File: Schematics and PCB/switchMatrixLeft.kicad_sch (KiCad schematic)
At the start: 151 parts, among them SW1 ESC, SW10 2, SW11 3, SW12 4, SW13 5, SW14 6, SW15 TAB, SW16 Q, SW17 W, SW18 E, SW19 R, SW2 F1, SW20 T, SW21 MAYUS, SW22 A, SW23 S, SW24 D, SW25 F, SW26 G, SW27 L_SHIFT, SW28 Z, SW29 X, SW3 F2, SW30 C, SW31 V, SW32 B, SW33 L_CRTL, SW34 OS, SW35 L_ALT, SW36 L_SPACE, SW4 F3, SW5 F4, SW6 F5, SW7 F6, SW8 `, SW9 1

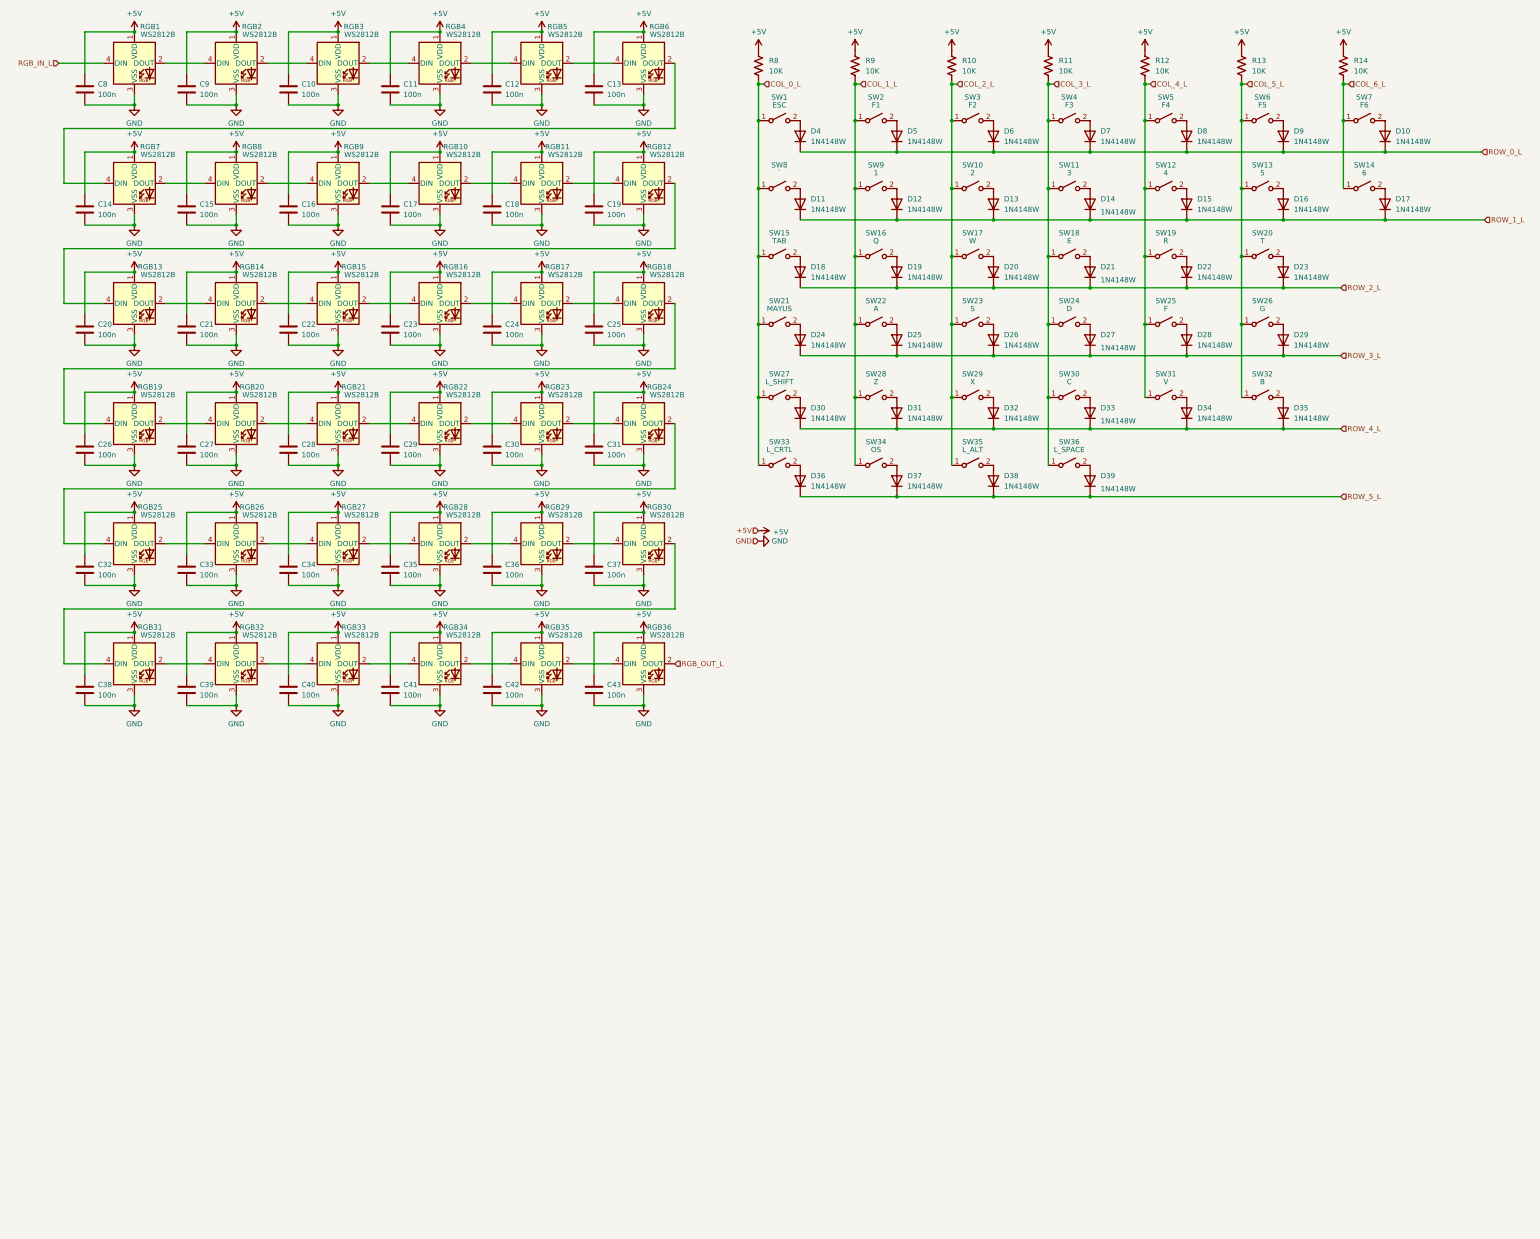
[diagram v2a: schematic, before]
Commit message: minor changes
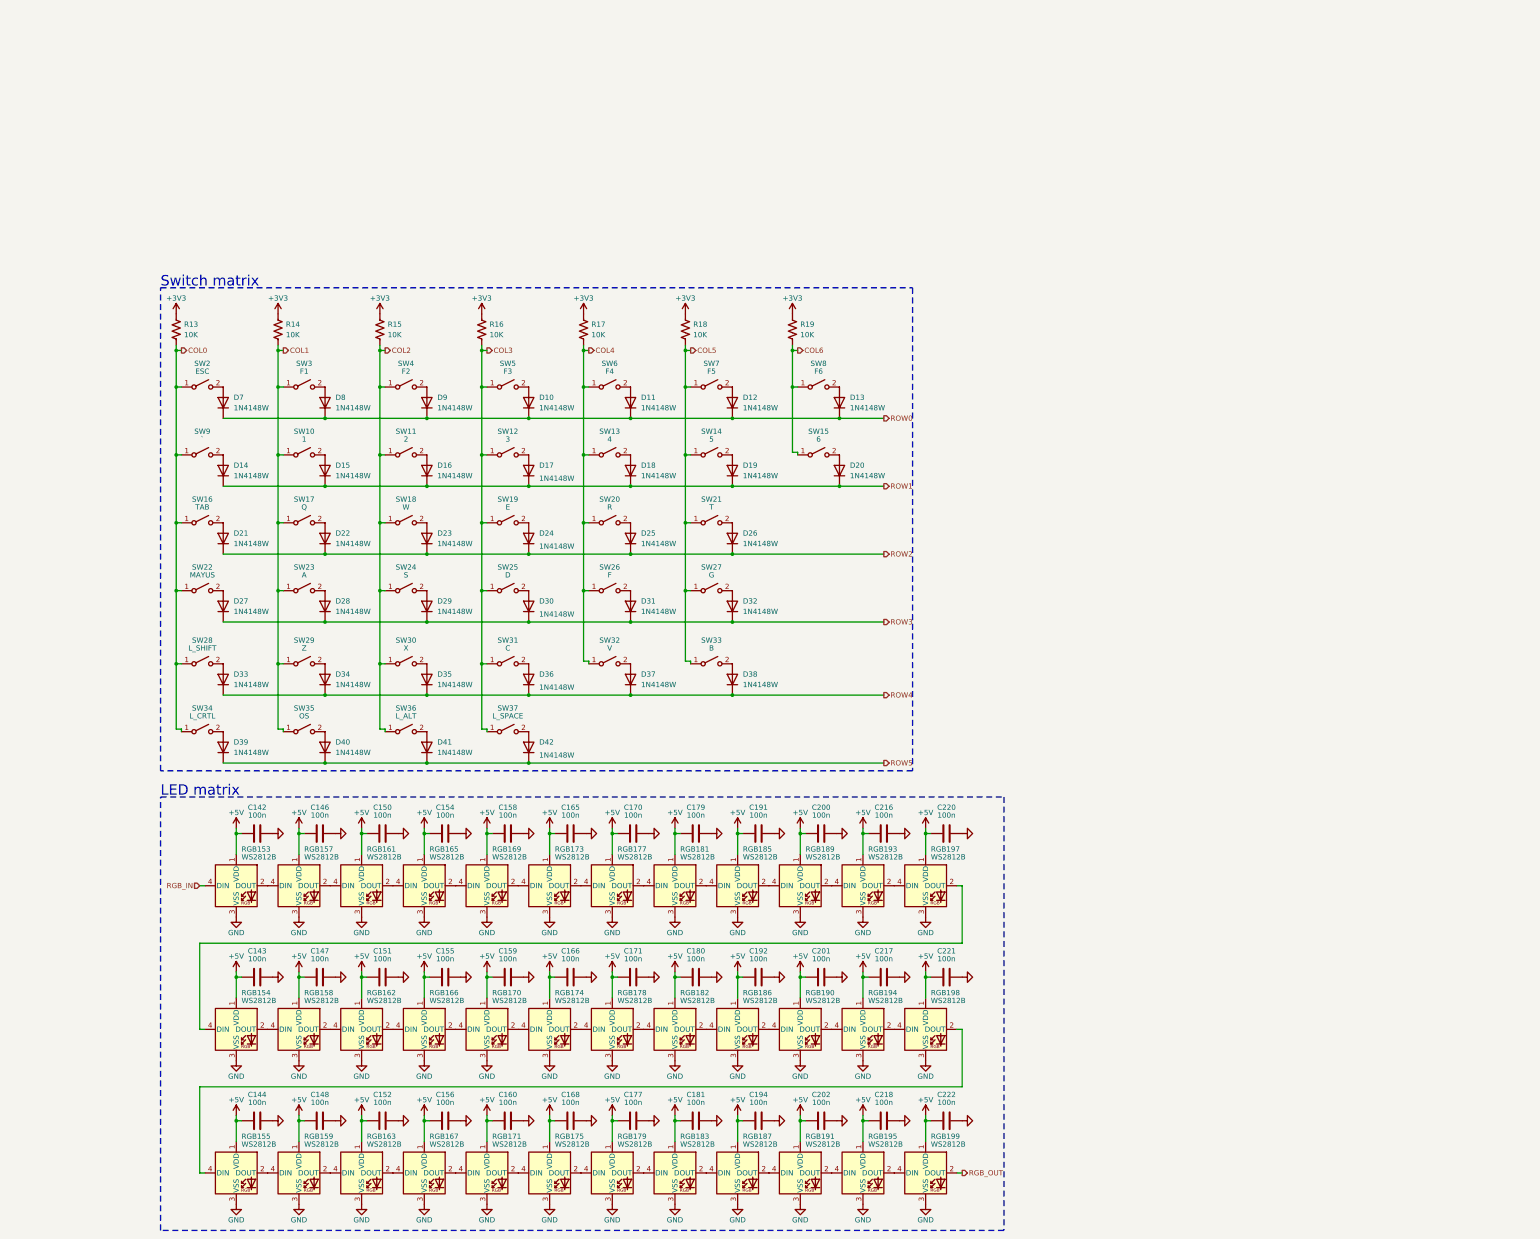
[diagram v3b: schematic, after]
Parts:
- removed C10, C11, C12, C13, C14, C15, C16, C17, C18, C19, C20, C21, C22, C23, C24, C25, C26, C27, C28, C29, C30, C31, C32, C33, C34, C35, C36, C37, C38, C39, C40, C41, C42, C43, C8, C9: 100n, Capacitor_SMD:C_0603_1608Metric, symbol Device:C
- removed RGB1, RGB10, RGB11, RGB12, RGB13, RGB14, RGB15, RGB16, RGB17, RGB18, RGB19, RGB2, RGB20, RGB21, RGB22, RGB23, RGB24, RGB25, RGB26, RGB27, RGB28, RGB29, RGB3, RGB30, RGB31, RGB32, RGB33, RGB34, RGB35, RGB36, RGB4, RGB5, RGB6, RGB7, RGB8, RGB9: WS2812B, LED_SMD:LED_WS2812B_PLCC4_5.0x5.0mm_P3.2mm, symbol LED:WS2812B
- added C142, C143, C144, C146, C147, C148, C150, C151, C152, C154, C155, C156, C158, C159, C160, C165, C166, C168, C170, C171, C177, C179, C180, C181, C191, C192, C194, C200, C201, C202, C216, C217, C218, C220, C221, C222: 100n, Capacitor_SMD:C_0805_2012Metric, symbol Device:C
- added RGB153, RGB154, RGB155, RGB157, RGB158, RGB159, RGB161, RGB162, RGB163, RGB165, RGB166, RGB167, RGB169, RGB170, RGB171, RGB173, RGB174, RGB175, RGB177, RGB178, RGB179, RGB181, RGB182, RGB183, RGB185, RGB186, RGB187, RGB189, RGB190, RGB191, RGB193, RGB194, RGB195, RGB197, RGB198, RGB199: WS2812B, LED_SMD:LED_WS2812B_PLCC4_5.0x5.0mm_P3.2mm, symbol LED:WS2812B
- renumbered D7 to D10, D8 to D11, D9 to D12, D10 to D13, D11 to D14, D12 to D15, D13 to D16, D14 to D17, D15 to D18, D16 to D19, D17 to D20, D18 to D21, D19 to D22, D20 to D23, D21 to D24, D22 to D25, D23 to D26, D24 to D27, D25 to D28, D26 to D29, D27 to D30, D28 to D31, D29 to D32, D30 to D33, D31 to D34, D32 to D35, D33 to D36, D34 to D37, D35 to D38, D36 to D39, D37 to D40, D38 to D41, D39 to D42, D4 to D7, D5 to D8, D6 to D9, R8 to R13, R9 to R14, R10 to R15, R11 to R16, R12 to R17, R13 to R18, R14 to R19, SW9 to SW10, SW10 to SW11, SW11 to SW12, SW12 to SW13, SW13 to SW14, SW14 to SW15, SW15 to SW16, SW16 to SW17, SW17 to SW18, SW18 to SW19, SW1 to SW2, SW19 to SW20, SW20 to SW21, SW21 to SW22, SW22 to SW23, SW23 to SW24, SW24 to SW25, SW25 to SW26, SW26 to SW27, SW27 to SW28, SW28 to SW29, SW2 to SW3, SW29 to SW30, SW30 to SW31, SW31 to SW32, SW32 to SW33, SW33 to SW34, SW34 to SW35, SW35 to SW36, SW36 to SW37, SW3 to SW4, SW4 to SW5, SW5 to SW6, SW6 to SW7, SW7 to SW8, SW8 to SW9
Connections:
- net +5V: now also C142.1, C143.1, C144.1, C146.1, C147.1, C148.1, C150.1, C151.1, C152.1, C154.1, C155.1, C156.1, C158.1, C159.1, C160.1, C165.1, C166.1, C168.1, C170.1, C171.1, C177.1, C179.1, C180.1, C181.1, C191.1, C192.1, C194.1, C200.1, C201.1, C202.1, C216.1, C217.1, C218.1, C220.1, C221.1, C222.1, RGB153.1 (VDD), RGB154.1 (VDD), RGB155.1 (VDD), RGB157.1 (VDD), RGB158.1 (VDD), RGB159.1 (VDD), RGB161.1 (VDD), RGB162.1 (VDD), RGB163.1 (VDD), RGB165.1 (VDD), RGB166.1 (VDD), RGB167.1 (VDD), RGB169.1 (VDD), RGB170.1 (VDD), RGB171.1 (VDD), RGB173.1 (VDD), RGB174.1 (VDD), RGB175.1 (VDD), RGB177.1 (VDD), RGB178.1 (VDD), RGB179.1 (VDD), RGB181.1 (VDD), RGB182.1 (VDD), RGB183.1 (VDD), RGB185.1 (VDD), RGB186.1 (VDD), RGB187.1 (VDD), RGB189.1 (VDD), RGB190.1 (VDD), RGB191.1 (VDD), RGB193.1 (VDD), RGB194.1 (VDD), RGB195.1 (VDD), RGB197.1 (VDD), RGB198.1 (VDD), RGB199.1 (VDD); no longer R13.1, R14.1, R15.1, R16.1, R17.1, R18.1, R19.1
- net GND: now also C142.2, C143.2, C144.2, C146.2, C147.2, C148.2, C150.2, C151.2, C152.2, C154.2, C155.2, C156.2, C158.2, C159.2, C160.2, C165.2, C166.2, C168.2, C170.2, C171.2, C177.2, C179.2, C180.2, C181.2, C191.2, C192.2, C194.2, C200.2, C201.2, C202.2, C216.2, C217.2, C218.2, C220.2, C221.2, C222.2, RGB153.3 (VSS), RGB154.3 (VSS), RGB155.3 (VSS), RGB157.3 (VSS), RGB158.3 (VSS), RGB159.3 (VSS), RGB161.3 (VSS), RGB162.3 (VSS), RGB163.3 (VSS), RGB165.3 (VSS), RGB166.3 (VSS), RGB167.3 (VSS), RGB169.3 (VSS), RGB170.3 (VSS), RGB171.3 (VSS), RGB173.3 (VSS), RGB174.3 (VSS), RGB175.3 (VSS), RGB177.3 (VSS), RGB178.3 (VSS), RGB179.3 (VSS), RGB181.3 (VSS), RGB182.3 (VSS), RGB183.3 (VSS), RGB185.3 (VSS), RGB186.3 (VSS), RGB187.3 (VSS), RGB189.3 (VSS), RGB190.3 (VSS), RGB191.3 (VSS), RGB193.3 (VSS), RGB194.3 (VSS), RGB195.3 (VSS), RGB197.3 (VSS), RGB198.3 (VSS), RGB199.3 (VSS)
- net COL_0_L renamed COL0
- net COL_1_L renamed COL1
- net COL_2_L renamed COL2
- net COL_3_L renamed COL3
- net COL_4_L renamed COL4
- net COL_5_L renamed COL5
- net COL_6_L renamed COL6
- net ROW_0_L renamed ROW0
- net ROW_1_L renamed ROW1
- net ROW_2_L renamed ROW2
- net ROW_3_L renamed ROW3
- net ROW_4_L renamed ROW4
- net ROW_5_L renamed ROW5
- new net: RGB174.2 (DOUT), RGB178.4 (DIN)
- new net: RGB170.2 (DOUT), RGB174.4 (DIN)
- new net: RGB154.2 (DOUT), RGB158.4 (DIN)
- new net: RGB154.4 (DIN), RGB197.2 (DOUT)
- new net: RGB161.2 (DOUT), RGB165.4 (DIN)
- new net: RGB157.2 (DOUT), RGB161.4 (DIN)
- new net: RGB153.2 (DOUT), RGB157.4 (DIN)
- new net: RGB191.2 (DOUT), RGB195.4 (DIN)
- new net: RGB187.2 (DOUT), RGB191.4 (DIN)
- new net: RGB185.2 (DOUT), RGB189.4 (DIN)
- new net: RGB181.2 (DOUT), RGB185.4 (DIN)
- new net: RGB165.2 (DOUT), RGB169.4 (DIN)
- new net: RGB155.4 (DIN), RGB198.2 (DOUT)
- new net: RGB194.2 (DOUT), RGB198.4 (DIN)
- new net: RGB155.2 (DOUT), RGB159.4 (DIN)
- new net: RGB190.2 (DOUT), RGB194.4 (DIN)
- new net: RGB186.2 (DOUT), RGB190.4 (DIN)
- new net: RGB182.2 (DOUT), RGB186.4 (DIN)
- new net: RGB178.2 (DOUT), RGB182.4 (DIN)
- new net: RGB169.2 (DOUT), RGB173.4 (DIN)
- new net: RGB166.2 (DOUT), RGB170.4 (DIN)
- new net: RGB162.2 (DOUT), RGB166.4 (DIN)
- new net: RGB163.2 (DOUT), RGB167.4 (DIN)
- new net: RGB159.2 (DOUT), RGB163.4 (DIN)
- new net: RGB193.2 (DOUT), RGB197.4 (DIN)
- new net: RGB179.2 (DOUT), RGB183.4 (DIN)
- new net: RGB175.2 (DOUT), RGB179.4 (DIN)
- new net: RGB171.2 (DOUT), RGB175.4 (DIN)
- new net: RGB167.2 (DOUT), RGB171.4 (DIN)
- new net: RGB177.2 (DOUT), RGB181.4 (DIN)
- new net: RGB183.2 (DOUT), RGB187.4 (DIN)
- new net: RGB195.2 (DOUT), RGB199.4 (DIN)
- new net: RGB173.2 (DOUT), RGB177.4 (DIN)
- new net: RGB189.2 (DOUT), RGB193.4 (DIN)
- new net: RGB158.2 (DOUT), RGB162.4 (DIN)
- new net +3V3: R13.1, R14.1, R15.1, R16.1, R17.1, R18.1, R19.1
- new net RGB_IN: RGB153.4 (DIN)
- new net RGB_OUT: RGB199.2 (DOUT)
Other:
- note added: "LED matrix"
- note added: "Switch matrix"
- moved on the sheet: D10, D11, D12, D13, D14, D15, D16, D17, D18, D19, D20, D21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
